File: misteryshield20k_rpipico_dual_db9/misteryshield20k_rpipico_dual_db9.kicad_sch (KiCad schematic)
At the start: 66 parts, among them J1 Joystick, J2 Joystick, J4 Conn_01x20_Pin, J5 Conn_01x02_Pin, J7 Conn_01x20_Pin, Q1 2N7002, Q10 2N7002, Q11 2N7002, Q12 2N7002, Q2 2N7002, Q3 2N7002, Q4 2N7002, Q5 2N7002, Q6 2N7002, Q7 2N7002, Q8 2N7002, Q9 2N7002, U1 USB_C_Receptacle_PowerOnly_6P

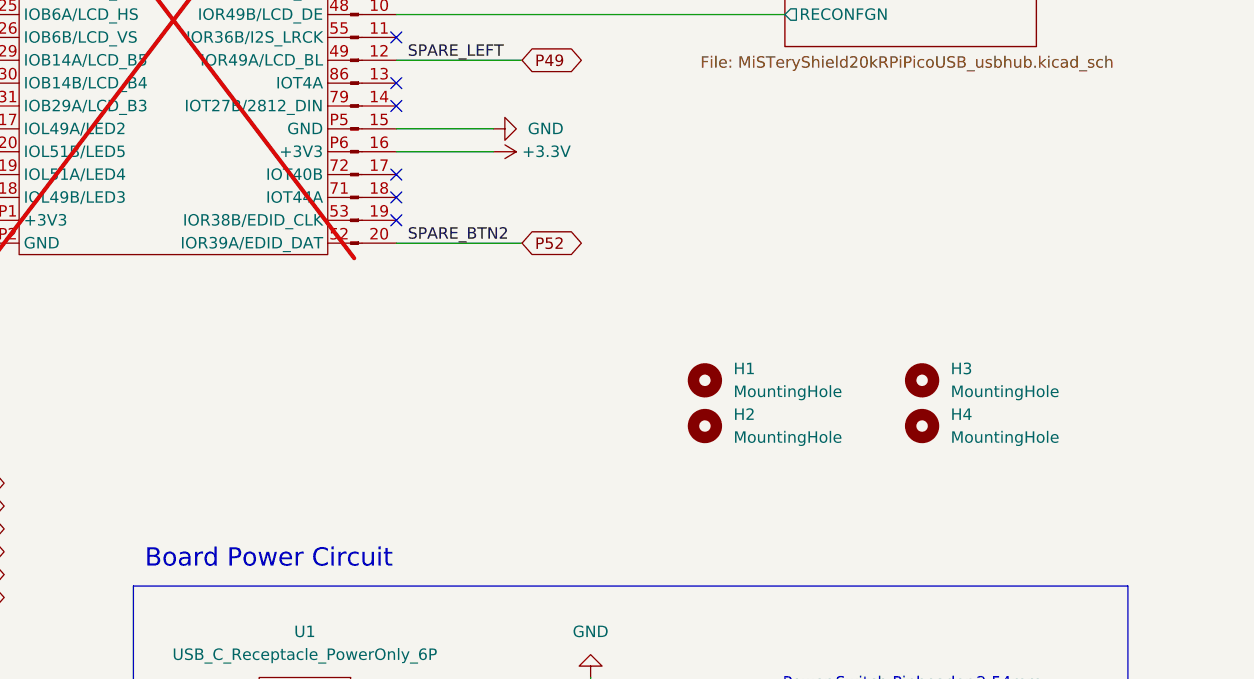
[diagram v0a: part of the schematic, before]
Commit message: Add files via upload
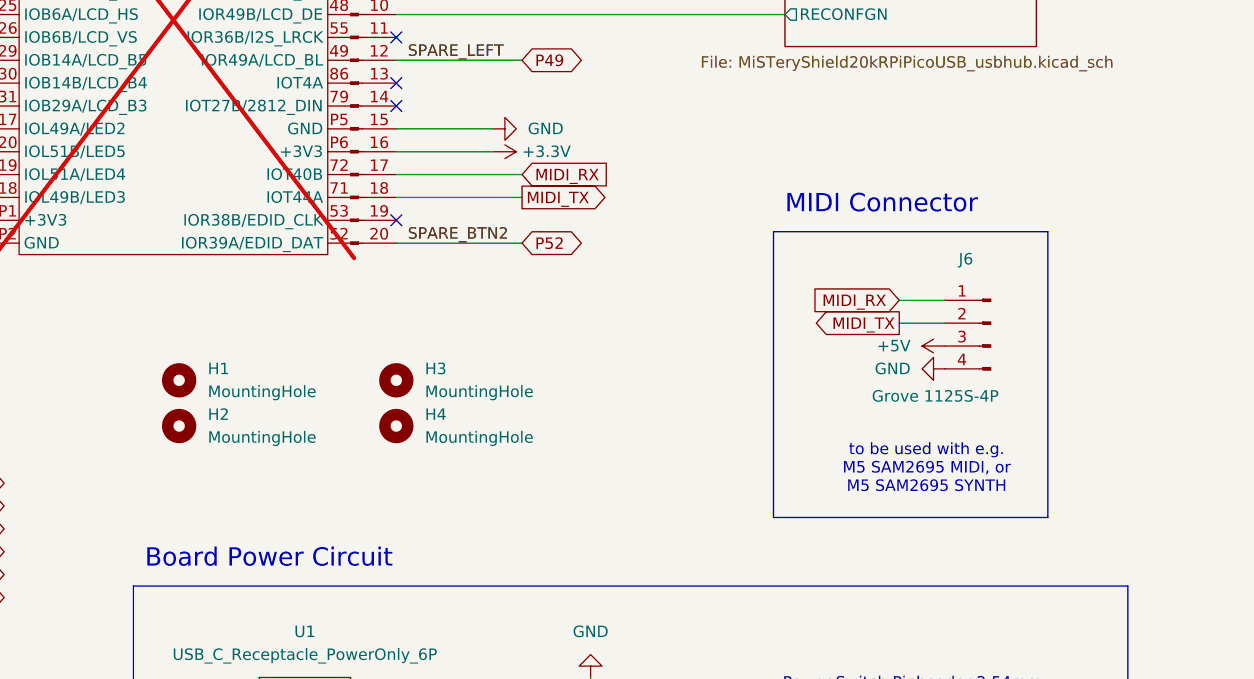
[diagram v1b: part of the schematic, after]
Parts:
- added J6: Grove 1125S-4P, Connector:NS-Tech_Grove_1x04_P2mm_Vertical, symbol Connector:Conn_01x04_Pin
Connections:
- net +5V: now also J6.3 (Pin_3)
- net GND: now also J6.4 (Pin_4)
- net MIDI_RX: now reaches J7.17 (Pin_17)
- net MIDI_RX: now also J6.1 (Pin_1)
- net MIDI_TX: now reaches J7.18 (Pin_18)
- net MIDI_TX: now also J6.2 (Pin_2)
- no-connect marks 14 -> 12
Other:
- note added: "MIDI Connector"
- note added: "to be used with e.g. M5 SAM2695 MIDI, or M5 SAM2695 SYNTH"
- moved on the sheet: H1, H2, H3, H4
